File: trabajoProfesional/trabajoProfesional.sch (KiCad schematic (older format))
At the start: 5 parts

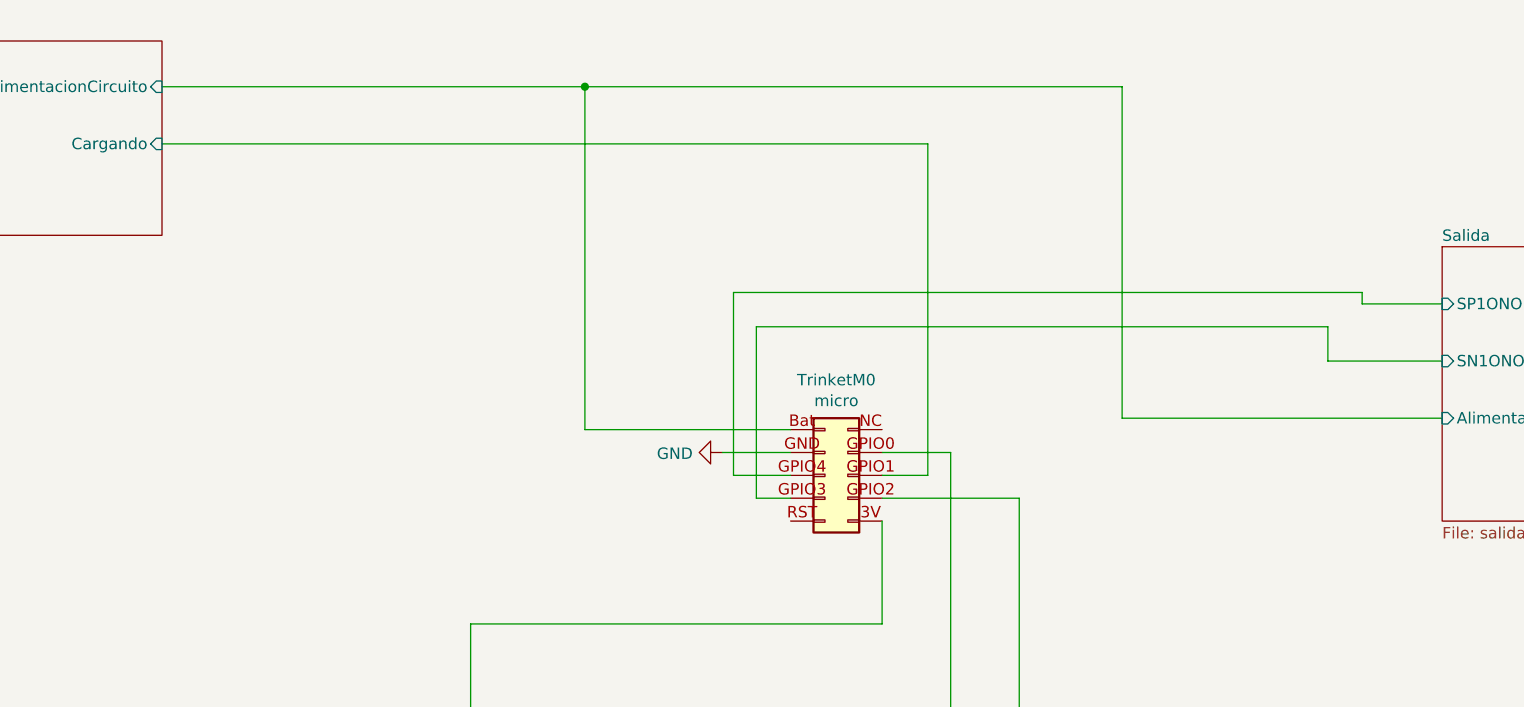
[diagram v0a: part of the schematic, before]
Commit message: paso previo PCB
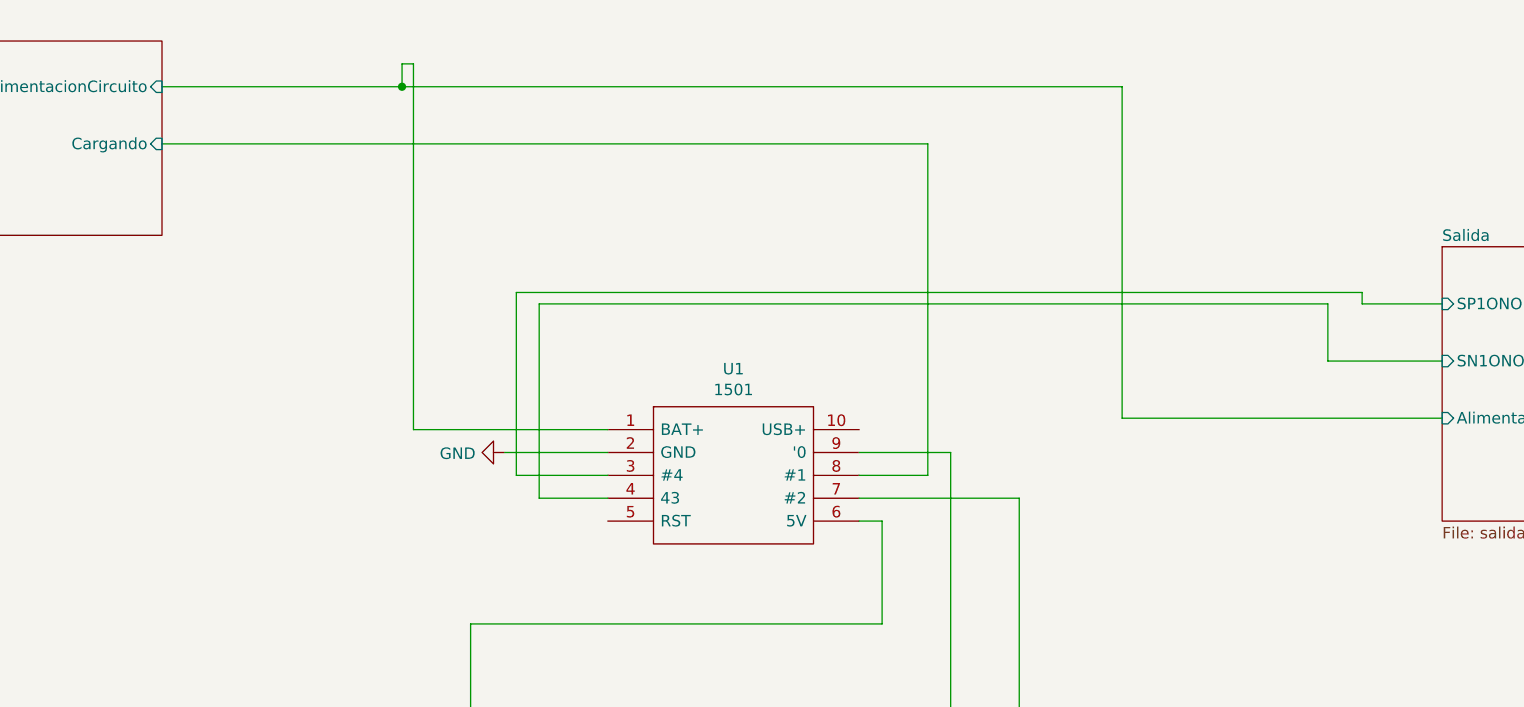
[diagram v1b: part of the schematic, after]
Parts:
- removed TrinketM0: micro, Connector_PinHeader_1.00mm:PinHeader_2x05_P1.00mm_Vertical, symbol Connector_Generic:Conn_02x05_Row_Letter_First
- added U1: 1501, Connector_PinHeader_1.00mm:PinHeader_2x05_P1.00mm_Vertical, symbol Trinket:1501
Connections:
- net Bateria/AlimentacionCircuito: now also U1.1 (BAT+)
- net Bateria/Cargando: now also U1.8 (#1)
- net GND: now also U1.2 (GND)
- net SCLPresion: now also U1.7 (#2)
- net SDAPresion: now also U1.9 ('0)
- net Salida/SN1ONOFF: now also U1.4 (43)
- net Salida/SP1ONOFF: now also U1.3 (#4)
- net at C6.2, R1.1, R2.1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: now also U1.6 (5V)
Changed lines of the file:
@@
 F3 "Cargando" I R 2350 1300 50
 $EndSheet
-$Comp
-L Connector_Generic:Conn_02x05_Row_Letter_First TrinketM0
-U 1 1 5F3DA13B
-P 5250 2750
-F 0 "TrinketM0" H 5300 3167 50  0000 C CNN
-F 1 "micro" H 5300 3076 50  0000 C CNN
-F 2 "Connector_PinHeader_1.00mm:PinHeader_2x05_P1.00mm_Vertical" H 5250 2750 50  0001 C CNN
-F 3 "~" H 5250 2750 50  0001 C CNN
-	1    5250 2750
-	1    0    0    -1
-$EndComp
-Wire Wire Line
-	5100 2550 4200 2550
-Wire Wire Line
-	4200 2550 4200 1050
 Wire Wire Line
 	7950 2500 6550 2500
 Wire Wire Line
 	6550 2500 6550 1050
-Wire Wire Line
-	6550 1050 4200 1050
-Connection ~ 4200 1050
 $Comp
 L power:GND #PWR0101
 U 1 1 5F3F217F
-P 4800 2650
-F 0 "#PWR0101" H 4800 2400 50  0001 C CNN
-F 1 "GND" V 4805 2522 50  0000 R CNN
-F 2 "" H 4800 2650 50  0001 C CNN
-F 3 "" H 4800 2650 50  0001 C CNN
-	1    4800 2650
+P 3850 2650
+F 0 "#PWR0101" H 3850 2400 50  0001 C CNN
+F 1 "GND" V 3855 2522 50  0000 R CNN
+F 2 "" H 3850 2650 50  0001 C CNN
+F 3 "" H 3850 2650 50  0001 C CNN
+	1    3850 2650
 	0    1    1    0
 $EndComp
-Wire Wire Line
-	5100 2650 4800 2650
-Wire Wire Line
-	2350 1050 4200 1050
 Wire Wire Line
 	5500 2950 5500 3400
@@
 Wire Wire Line
 	6100 4550 6100 2850
-Wire Wire Line
-	6100 2850 5500 2850
 Connection ~ 6100 4550
 Wire Wire Line
@@
 Wire Wire Line
 	5800 3950 5800 2650
-Wire Wire Line
-	5800 2650 5500 2650
 Connection ~ 4800 4200
 Wire Wire Line
 	4800 4200 4900 4200
 Wire Wire Line
-	5100 2750 4850 2750
-Wire Wire Line
-	4850 2750 4850 1950
-Wire Wire Line
-	4850 1950 7600 1950
+	3900 2750 3900 1950
 Wire Wire Line
 	7600 1950 7600 2000
@@
 	7600 2000 7950 2000
 Wire Wire Line
-	5100 2850 4950 2850
-Wire Wire Line
-	4950 2850 4950 2100
-Wire Wire Line
-	4950 2100 7450 2100
-Wire Wire Line
-	7450 2100 7450 2250
-Wire Wire Line
 	7450 2250 7950 2250
-Wire Wire Line
-	5500 2750 5700 2750
 Wire Wire Line
 	5700 2750 5700 1300
 Wire Wire Line
 	5700 1300 2350 1300
+$Comp
+L Trinket:1501 U1
+U 1 1 5F3DB5D3
+P 4300 2550
+F 0 "U1" H 4850 2815 50  0000 C CNN
+F 1 "1501" H 4850 2724 50  0000 C CNN
+F 2 "Connector_PinHeader_1.00mm:PinHeader_2x05_P1.00mm_Vertical" H 5250 2650 50  0001 L CNN
+F 3 "https://learn.adafruit.com/introducing-trinket" H 5250 2550 50  0001 L CNN
+F 4 "ADAFRUIT - 1501 - TRINKET DEV BOARD, ATTINY85 MCU, 5V" H 5250 2450 50  0001 L CNN "Description"
+F 5 "" H 5250 2350 50  0001 L CNN "Height"
+F 6 "Adafruit" H 5250 2250 50  0001 L CNN "Manufacturer_Name"
+F 7 "1501" H 5250 2150 50  0001 L CNN "Manufacturer_Part_Number"
+F 8 "1501" H 5250 2050 50  0001 L CNN "Arrow Part Number"
+F 9 "https://www.arrow.com/en/products/1501/adafruit-industries" H 5250 1950 50  0001 L CNN "Arrow Price/Stock"
+F 10 "485-1501" H 5250 1850 50  0001 L CNN "Mouser Part Number"
+F 11 "https://www.mouser.co.uk/ProductDetail/Adafruit/1501?qs=GURawfaeGuApEwtfdnWm9A%3D%3D" H 5250 1750 50  0001 L CNN "Mouser Price/Stock"
+	1    4300 2550
+	1    0    0    -1
+$EndComp
+Wire Wire Line
+	2350 1050 3400 1050
+Wire Wire Line
+	5400 2650 5800 2650
+Wire Wire Line
+	5400 2750 5700 2750
+Wire Wire Line
+	5400 2850 6100 2850
+Wire Wire Line
+	5500 2950 5400 2950
+Wire Wire Line
+	3850 2650 4300 2650
+Wire Wire Line
+	3900 2750 4300 2750
+Wire Wire Line
+	4000 2850 4300 2850
+Wire Wire Line
+	3900 1950 7600 1950
+Wire Wire Line
+	4000 2000 4000 2850
+Wire Wire Line
+	7450 2000 7450 2250
+Wire Wire Line
+	4000 2000 7450 2000
+Wire Wire Line
+	3450 950  3450 2550
+Wire Wire Line
+	3450 2550 4300 2550
+Wire Wire Line
+	3400 1050 3400 950
+Wire Wire Line
+	3400 950  3450 950
+Connection ~ 3400 1050
+Wire Wire Line
+	3400 1050 6550 1050
 $EndSCHEMATC

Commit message: va el circuito
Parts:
- C6: footprint Capacitor_SMD:C_2816_7142Metric -> Capacitor_SMD:C_0201_0603Metric
- R1, R2: footprint Resistor_SMD:R_1206_3216Metric -> Resistor_SMD:R_0201_0603Metric
- SensorPresion1: footprint Connector_PinSocket_2.54mm:PinSocket_2x02_P2.54mm_Vertical_SMD -> Connector_PinHeader_2.54mm:PinHeader_2x02_P2.54mm_Vertical
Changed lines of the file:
@@
 F 0 "SensorPresion1" H 5050 6687 60  0000 C CNN
 F 1 "MS583730BA01-50" H 5050 6581 60  0000 C CNN
-F 2 "Connector_PinSocket_2.54mm:PinSocket_2x02_P2.54mm_Vertical_SMD" H 5050 6540 60  0001 C CNN
+F 2 "Connector_PinHeader_2.54mm:PinHeader_2x02_P2.54mm_Vertical" H 5050 6540 60  0001 C CNN
 F 3 "" H 4250 6300 60  0000 C CNN
 	1    4250 6300
@@
 F 0 "C6" V 4748 5700 50  0000 C CNN
 F 1 "100n" V 4839 5700 50  0000 C CNN
-F 2 "Capacitor_SMD:C_2816_7142Metric" H 5038 5550 50  0001 C CNN
+F 2 "Capacitor_SMD:C_0201_0603Metric" H 5038 5550 50  0001 C CNN
 F 3 "~" H 5000 5700 50  0001 C CNN
 	1    5000 5700
@@
 F 0 "R1" H 3470 6246 50  0000 L CNN
 F 1 "10k" H 3470 6155 50  0000 L CNN
-F 2 "Resistor_SMD:R_1206_3216Metric" V 3330 6200 50  0001 C CNN
+F 2 "Resistor_SMD:R_0201_0603Metric" V 3330 6200 50  0001 C CNN
 F 3 "~" H 3400 6200 50  0001 C CNN
 	1    3400 6200
@@
 F 0 "R2" H 3220 6246 50  0000 L CNN
 F 1 "10k" H 3220 6155 50  0000 L CNN
-F 2 "Resistor_SMD:R_1206_3216Metric" V 3080 6200 50  0001 C CNN
+F 2 "Resistor_SMD:R_0201_0603Metric" V 3080 6200 50  0001 C CNN
 F 3 "~" H 3150 6200 50  0001 C CNN
 	1    3150 6200
